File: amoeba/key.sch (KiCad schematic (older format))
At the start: 0 parts

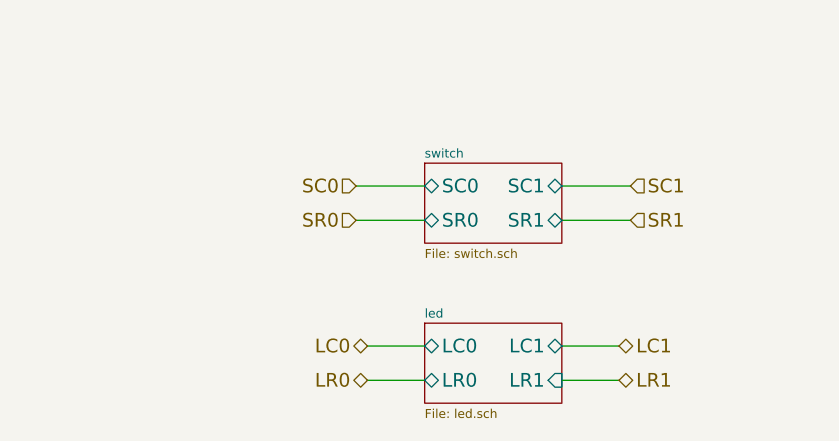
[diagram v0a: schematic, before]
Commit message: Schematic clean-up.
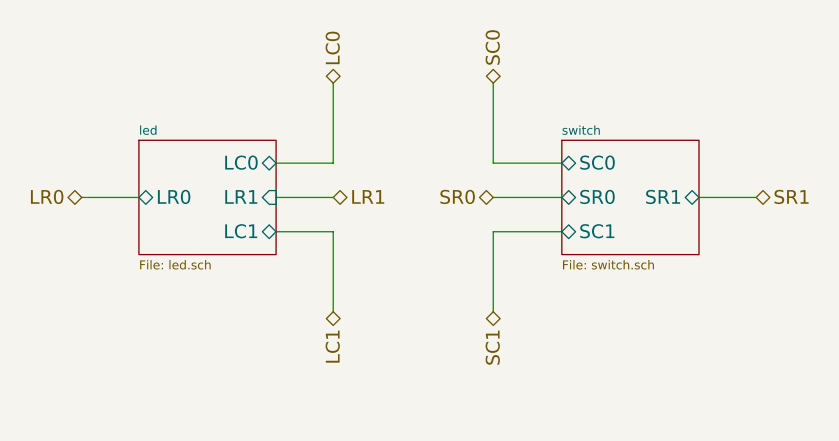
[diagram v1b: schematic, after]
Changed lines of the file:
@@
 Comment4 ""
 $EndDescr
-Text HLabel 5550 4100 0    60   BiDi ~ 0
+Text HLabel 5400 2950 1    60   BiDi ~ 0
 LC0
-Text HLabel 6650 4250 2    60   BiDi ~ 0
+Text HLabel 5400 3450 2    60   BiDi ~ 0
 LR1
-Text HLabel 5550 4250 0    60   BiDi ~ 0
+Text HLabel 4300 3450 0    60   BiDi ~ 0
 LR0
-Text HLabel 6650 4100 2    60   BiDi ~ 0
+Text HLabel 5400 3950 3    60   BiDi ~ 0
 LC1
 $Sheet
-S 5800 4000 600  350
+S 4550 3200 600  500
 U 55DBAE59
 F0 "led" 39
 F1 "led.sch" 39
-F2 "LC0" B L 5800 4100 60
-F3 "LR0" B L 5800 4250 60
-F4 "LC1" B R 6400 4100 60
-F5 "LR1" I R 6400 4250 60
+F2 "LC0" B R 5150 3300 60
+F3 "LR0" B L 4550 3450 60
+F4 "LC1" B R 5150 3600 60
+F5 "LR1" I R 5150 3450 60
 $EndSheet
 $Sheet
-S 5800 3300 600  350
+S 6400 3200 600  500
 U 55DBAE5B
 F0 "switch" 39
 F1 "switch.sch" 39
-F2 "SC0" B L 5800 3400 60
-F3 "SR1" B R 6400 3550 60
-F4 "SR0" B L 5800 3550 60
-F5 "SC1" B R 6400 3400 60
+F2 "SC0" B L 6400 3300 60
+F3 "SR1" B R 7000 3450 60
+F4 "SR0" B L 6400 3450 60
+F5 "SC1" B L 6400 3600 60
 $EndSheet
 Wire Wire Line
-	6650 4100 6400 4100
-Wire Wire Line
-	6400 4250 6650 4250
-Wire Wire Line
-	5800 4250 5550 4250
-Wire Wire Line
-	5550 4100 5800 4100
-Text HLabel 5500 3400 0    60   Input ~ 0
+	4550 3450 4300 3450
+Text HLabel 6100 2950 1    60   BiDi ~ 0
 SC0
-Text HLabel 6700 3400 2    60   Input ~ 0
+Text HLabel 6100 3950 3    60   BiDi ~ 0
 SC1
-Text HLabel 6700 3550 2    60   Input ~ 0
+Text HLabel 7250 3450 2    60   BiDi ~ 0
 SR1
-Text HLabel 5500 3550 0    60   Input ~ 0
+Text HLabel 6100 3450 0    60   BiDi ~ 0
 SR0
 Wire Wire Line
-	6700 3400 6400 3400
+	6400 3450 6100 3450
 Wire Wire Line
-	6400 3550 6700 3550
+	5150 3300 5400 3300
 Wire Wire Line
-	5800 3550 5500 3550
+	5400 3300 5400 2950
 Wire Wire Line
-	5500 3400 5800 3400
+	5150 3450 5400 3450
+Wire Wire Line
+	5150 3600 5400 3600
+Wire Wire Line
+	5400 3600 5400 3950
+Wire Wire Line
+	7250 3450 7000 3450
+Wire Wire Line
+	6400 3300 6100 3300
+Wire Wire Line
+	6100 3300 6100 2950
+Wire Wire Line
+	6100 3950 6100 3600
+Wire Wire Line
+	6100 3600 6400 3600
 $EndSCHEMATC
